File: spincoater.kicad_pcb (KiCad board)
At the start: 2 copper layers, 100 x 60 mm, 1 part, among them U301 TMC4671-ES

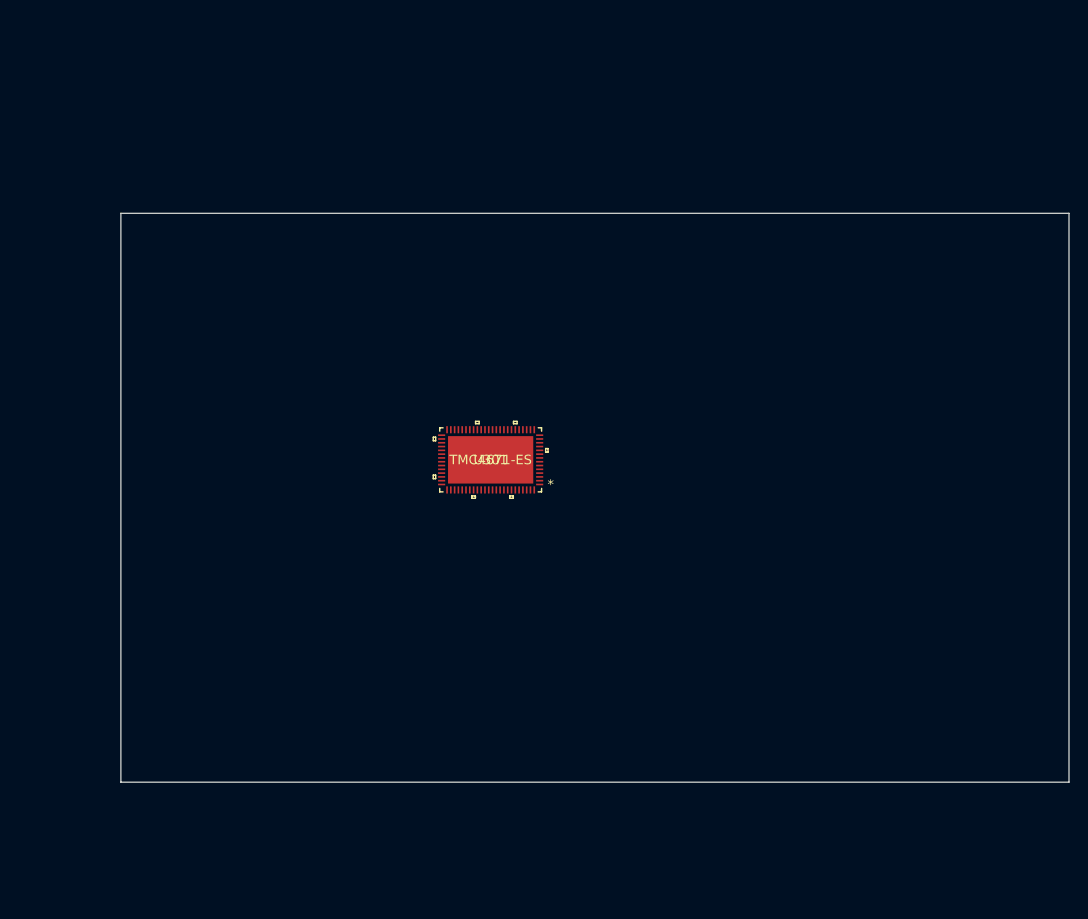
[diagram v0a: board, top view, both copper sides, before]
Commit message: antes de comenzar a rutear
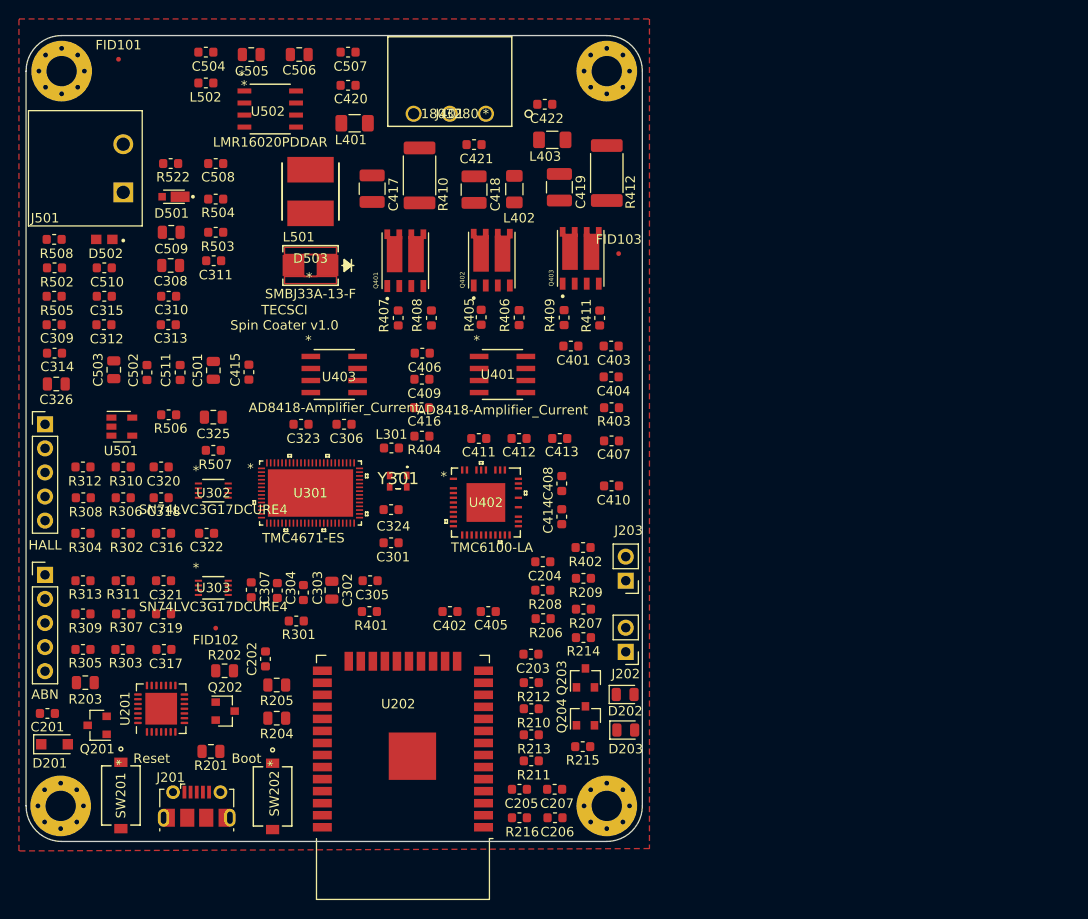
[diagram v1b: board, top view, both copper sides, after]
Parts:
- added C201: 0.1uF/50V/0603, Capacitor_SMD:C_0603_1608Metric, F.Cu at (42.2, 111.8)
- added C202: 0.1uF/50V/0603, Capacitor_SMD:C_0603_1608Metric, F.Cu at (65.2, 106.0)
- added C203: 100nF/50V/0603, Capacitor_SMD:C_0603_1608Metric, F.Cu at (93.2, 105.5)
- added C204: 100nF/50V/0603, Capacitor_SMD:C_0603_1608Metric, F.Cu at (94.5, 95.8)
- added C205: 0.1uF/50V/0603, Capacitor_SMD:C_0603_1608Metric, F.Cu at (92.0, 119.8)
- added C206: 22uF/10V/0603, Capacitor_SMD:C_0603_1608Metric, F.Cu at (95.8, 122.8)
- added C207: 0.1uF/50V/0603, Capacitor_SMD:C_0603_1608Metric, F.Cu at (95.8, 119.8)
- added C301: 100nF/50V/0603, Capacitor_SMD:C_0603_1608Metric, F.Cu at (78.5, 93.8)
- added C302: 4.7uF/16V/0805, Capacitor_SMD:C_0805_2012Metric, F.Cu at (72.2, 98.8)
- added C303: 100nF/50V/0603, Capacitor_SMD:C_0603_1608Metric, F.Cu at (69.2, 99.0)
- added C304: 100nF/50V/0603, Capacitor_SMD:C_0603_1608Metric, F.Cu at (66.5, 98.8)
- added C305: 100nF/50V/0603, Capacitor_SMD:C_0603_1608Metric, F.Cu at (76.3, 97.8)
- added C306: 100nF/50V/0603, Capacitor_SMD:C_0603_1608Metric, F.Cu at (73.5, 81.2)
- added C307: 100nF/50V/0603, Capacitor_SMD:C_0603_1608Metric, F.Cu at (63.8, 98.7)
- added C308: 4.7uF/16V/0805, Capacitor_SMD:C_0805_2012Metric, F.Cu at (55.2, 64.5)
- added C309: 470nF/50V/0603, Capacitor_SMD:C_0603_1608Metric, F.Cu at (43.0, 70.8)
- added C310: 100nF/50V/0603, Capacitor_SMD:C_0603_1608Metric, F.Cu at (55.0, 67.8)
- added C311: 100nF/50V/0603, Capacitor_SMD:C_0603_1608Metric, F.Cu at (59.8, 64.0)
- added C312: 100nF/50V/0603, Capacitor_SMD:C_0603_1608Metric, F.Cu at (48.2, 70.8)
- added C313: 100nF/50V/0603, Capacitor_SMD:C_0603_1608Metric, F.Cu at (55.0, 70.8)
- added C314: 100nF/50V/0603, Capacitor_SMD:C_0603_1608Metric, F.Cu at (43.0, 73.8)
- added C315: 100nF/50V/0603, Capacitor_SMD:C_0603_1608Metric, F.Cu at (48.2, 67.8)
- added C316: 1nF/100V/0603, Capacitor_SMD:C_0603_1608Metric, F.Cu at (54.5, 92.8)
- added C317: 1nF/100V/0603, Capacitor_SMD:C_0603_1608Metric, F.Cu at (54.5, 105.0)
- added C318: 1nF/100V/0603, Capacitor_SMD:C_0603_1608Metric, F.Cu at (54.2, 89.0)
- added C319: 1nF/100V/0603, Capacitor_SMD:C_0603_1608Metric, F.Cu at (54.5, 101.2)
- added C320: 1nF/100V/0603, Capacitor_SMD:C_0603_1608Metric, F.Cu at (54.2, 85.8)
- added C321: 1nF/100V/0603, Capacitor_SMD:C_0603_1608Metric, F.Cu at (54.5, 97.8)
- added C322: 100nF/50V/0603, Capacitor_SMD:C_0603_1608Metric, F.Cu at (59.0, 92.8)
- added C323: 100nF/50V/0603, Capacitor_SMD:C_0603_1608Metric, F.Cu at (69.0, 81.2)
- added C324: 100nF/50V 0603, Capacitor_SMD:C_0603_1608Metric, F.Cu at (78.5, 90.2)
- added C325: 1uF/50V/0805, Capacitor_SMD:C_0805_2012Metric, F.Cu at (59.8, 80.5)
- added C326: 1uF/50V/0805, Capacitor_SMD:C_0805_2012Metric, F.Cu at (43.2, 77.0)
- added C401: 100nF/50v/0603, Capacitor_SMD:C_0603_1608Metric, F.Cu at (97.5, 73.0)
- added C402: 2.2uF/16V/0603, Capacitor_SMD:C_0603_1608Metric, F.Cu at (84.7, 101.0)
- added C403: 2.2uF/16V/0603, Capacitor_SMD:C_0603_1608Metric, F.Cu at (101.7, 73.0)
- added C404: 100nF/50V/0603, Capacitor_SMD:C_0603_1608Metric, F.Cu at (101.7, 76.2)
- added C405: 100nF/50V/0603, Capacitor_SMD:C_0603_1608Metric, F.Cu at (88.8, 101.0)
- added C406: 100nF/50V/0603, Capacitor_SMD:C_0603_1608Metric, F.Cu at (81.8, 73.8)
- added C407: 2.2nF/50V/0603, Capacitor_SMD:C_0603_1608Metric, F.Cu at (101.8, 83.0)
- added C408: 100nF/50V/0603, Capacitor_SMD:C_0603_1608Metric, F.Cu at (96.5, 87.5)
- added C409: 100nF/50V/0603, Capacitor_SMD:C_0603_1608Metric, F.Cu at (81.8, 76.5)
- added C410: 100nF/50V/0603, Capacitor_SMD:C_0603_1608Metric, F.Cu at (101.8, 87.8)
- added C411: 470nF/50V/0603, Capacitor_SMD:C_0603_1608Metric, F.Cu at (87.8, 82.8)
- added C412: 470nF/50V/0603, Capacitor_SMD:C_0603_1608Metric, F.Cu at (92.0, 82.8)
- added C413: 470nF/50V/0603, Capacitor_SMD:C_0603_1608Metric, F.Cu at (96.3, 82.8)
- added C414: 22nF/100V/0603, Capacitor_SMD:C_0603_1608Metric, F.Cu at (96.5, 91.0)
- added C415: 100nF/50V/0603, Capacitor_SMD:C_0603_1608Metric, F.Cu at (63.5, 75.8)
- added C416: 2.2nF/50V/0603, Capacitor_SMD:C_0603_1608Metric, F.Cu at (81.7, 79.5)
- added C417: 10uF/50V/1210, Capacitor_SMD:C_1210_3225Metric, F.Cu at (76.5, 56.4)
- added C418: 10uF/50V/1210, Capacitor_SMD:C_1210_3225Metric, F.Cu at (87.2, 56.5)
- added C419: 10uF/50V/1210, Capacitor_SMD:C_1210_3225Metric, F.Cu at (96.2, 56.2)
- added C420: 1nF/100V/0603, Capacitor_SMD:C_0603_1608Metric, F.Cu at (74.0, 45.5)
- added C421: 1nF/100V/0603, Capacitor_SMD:C_0603_1608Metric, F.Cu at (87.2, 51.8)
- added C422: 1nF/100V/0603, Capacitor_SMD:C_0603_1608Metric, F.Cu at (94.7, 47.5)
- added C501: 10uF/16V/0805, Capacitor_SMD:C_0805_2012Metric, F.Cu at (59.8, 75.6)
- added C502: 10nF/16V/0603, Capacitor_SMD:C_0603_1608Metric, F.Cu at (52.8, 75.8)
- added C503: 10uF/16V/0805, Capacitor_SMD:C_0805_2012Metric, F.Cu at (49.2, 75.5)
- added C504: 100nF/50V/0603, Capacitor_SMD:C_0603_1608Metric, F.Cu at (59.0, 42.0)
- added C505: 2.2uF/50V/0805, Capacitor_SMD:C_0805_2012Metric, F.Cu at (63.8, 42.2)
- added C506: 2.2uF/50V/0805, Capacitor_SMD:C_0805_2012Metric, F.Cu at (68.8, 42.2)
- added C507: 100nF/50V/0603, Capacitor_SMD:C_0603_1608Metric, F.Cu at (74.0, 42.0)
- added C508: 100nF/50V/0603, Capacitor_SMD:C_0603_1608Metric, F.Cu at (60.0, 53.8)
- added C509: 10uF/16V/0805, Capacitor_SMD:C_0805_2012Metric, F.Cu at (55.3, 61.0)
- added C510: 100nF/50V/0603, Capacitor_SMD:C_0603_1608Metric, F.Cu at (48.2, 64.8)
- added C511: 100nF/50V/0603, Capacitor_SMD:C_0603_1608Metric, F.Cu at (56.2, 75.8)
- added D201: PMEG3020EH, Diode_SMD:D_SOD-123F, F.Cu at (43.0, 115.0)
- added D202: LED, LED_SMD:LED_0805_2012Metric, F.Cu at (103.2, 109.8)
- added D203: LED, LED_SMD:LED_0805_2012Metric, F.Cu at (103.2, 113.5)
- added D501: V2PM10HM3, DIODE_MSS1P4-M3:DIODE_MSS1P4-M3, F.Cu at (55.6, 57.2)
- added D502: LTST-C191TBKT-5A, LTST-C191TBKT-5A:LTST-C191TBKT-5A, F.Cu at (48.2, 61.8)
- added D503: SMBJ33A-13-F, SMBJ33A-13-F:SMBJ33A-13-F, F.Cu at (70.0, 64.5)
- added FID101: Fiducial, Fiducial:Fiducial_0.5mm_Mask1mm, F.Cu at (49.8, 42.8)
- added FID102: Fiducial, Fiducial:Fiducial_0.5mm_Mask1mm, F.Cu at (60.0, 102.8)
- added FID103: Fiducial, Fiducial:Fiducial_0.5mm_Mask1mm, F.Cu at (102.5, 63.2)
- added H101: MountingHole_Pad, MountingHole:MountingHole_3.2mm_M3_Pad_Via, F.Cu at (43.8, 44.0)
- added H102: MountingHole_Pad, MountingHole:MountingHole_3.2mm_M3_Pad_Via, F.Cu at (43.6, 121.5)
- added H103: MountingHole_Pad, MountingHole:MountingHole_3.2mm_M3_Pad_Via, F.Cu at (101.2, 121.5)
- added H104: MountingHole_Pad, MountingHole:MountingHole_3.2mm_M3_Pad_Via, F.Cu at (101.2, 44.0)
- added J201: USB_B_Micro, Connector_USB:USB_Micro-B_Molex-105017-0001, F.Cu at (58.0, 121.5)
- added J202: Conn_01x02, Connector_PinHeader_2.54mm:PinHeader_1x02_P2.54mm_Vertical, F.Cu at (103.2, 105.2)
- added J203: Conn_01x02, Connector_PinHeader_2.54mm:PinHeader_1x02_P2.54mm_Vertical, F.Cu at (103.2, 97.8)
- added J301: Conn_01x05, Connector_PinHeader_2.54mm:PinHeader_1x05_P2.54mm_Vertical, F.Cu at (42.0, 81.2)
- added J302: Conn_01x05, Connector_PinHeader_2.54mm:PinHeader_1x05_P2.54mm_Vertical, F.Cu at (42.0, 97.1)
- added J401: 1803280, 1803280:1803280, F.Cu at (88.5, 48.5)
- added J501: 1757242, PHOENIX_1757242:PHOENIX_1757242, F.Cu at (46.2, 54.2)
- added L301: 600R/1A/0603, Inductor_SMD:L_0603_1608Metric, F.Cu at (78.5, 83.8)
- added L401: 50R/12A/1206, Inductor_SMD:L_1206_3216Metric, F.Cu at (74.7, 49.5)
- added L402: 50R/12A/1206, Inductor_SMD:L_1206_3216Metric, F.Cu at (91.5, 56.5)
- added L403: 50R/12A/1206, Inductor_SMD:L_1206_3216Metric, F.Cu at (95.5, 51.2)
- added L501: 15uH/2.5A/VLS6045, INDPM6060X450N:INDPM6060X450N, F.Cu at (70.0, 56.7)
- added L502: 600R/1A/0603, Inductor_SMD:L_0603_1608Metric, F.Cu at (59.0, 45.2)
- added Q201: S8050, Package_TO_SOT_SMD:SOT-23, F.Cu at (47.5, 113.0)
- added Q202: S8050, Package_TO_SOT_SMD:SOT-23, F.Cu at (61.0, 111.5)
- added Q203: 2N7002, Package_TO_SOT_SMD:SOT-23, F.Cu at (99.0, 108.0)
- added Q204: 2N7002, Package_TO_SOT_SMD:SOT-23, F.Cu at (99.0, 112.0)
- added Q401: SI7288DP-T1-GE3, SI7288DP-T1-GE3:TRANS_SI7288DP-T1-GE3, F.Cu at (80.0, 64.0)
- added Q402: SI7288DP-T1-GE3, SI7288DP-T1-GE3:TRANS_SI7288DP-T1-GE3, F.Cu at (89.1, 63.9)
- added Q403: SI7288DP-T1-GE3, SI7288DP-T1-GE3:TRANS_SI7288DP-T1-GE3, F.Cu at (98.5, 63.8)
- added R201: 4.7K/1%/0805, Resistor_SMD:R_0805_2012Metric, F.Cu at (59.5, 115.8)
- added R202: 10K/1%/0805, Resistor_SMD:R_0805_2012Metric, F.Cu at (60.9, 107.2)
- added R203: 10K/1%/0805, Resistor_SMD:R_0805_2012Metric, F.Cu at (46.2, 108.5)
- added R204: 1K/1%/0805, Resistor_SMD:R_0805_2012Metric, F.Cu at (66.4, 112.2)
- added R205: 1K/1%/0805, Resistor_SMD:R_0805_2012Metric, F.Cu at (66.4, 108.8)
- added R206: 1K/1%/0603, Resistor_SMD:R_0603_1608Metric, F.Cu at (94.5, 101.8)
- added R207: 10K/1%/0603, Resistor_SMD:R_0603_1608Metric, F.Cu at (98.8, 100.8)
- added R208: 1K/1%/0603, Resistor_SMD:R_0603_1608Metric, F.Cu at (94.5, 98.8)
- added R209: 10K/1%/0603, Resistor_SMD:R_0603_1608Metric, F.Cu at (98.8, 97.5)
- added R210: 330K/1%/0603, Resistor_SMD:R_0603_1608Metric, F.Cu at (93.3, 111.2)
- added R211: 330K/1%/0603, Resistor_SMD:R_0603_1608Metric, F.Cu at (93.3, 116.8)
- added R212: 10K/1%/0603, Resistor_SMD:R_0603_1608Metric, F.Cu at (93.3, 108.5)
- added R213: 10K/1%/0603, Resistor_SMD:R_0603_1608Metric, F.Cu at (93.3, 114.0)
- added R214: 680/1%/0603, Resistor_SMD:R_0603_1608Metric, F.Cu at (98.8, 103.8)
- added R215: 680/1%/0603, Resistor_SMD:R_0603_1608Metric, F.Cu at (98.7, 115.2)
- added R216: 10K/1%/0603, Resistor_SMD:R_0603_1608Metric, F.Cu at (92.0, 122.8)
- added R301: 10K/1%/0603, Resistor_SMD:R_0603_1608Metric, F.Cu at (68.5, 102.0)
- added R302: 4K7/1%/0603, Resistor_SMD:R_0603_1608Metric, F.Cu at (50.2, 92.8)
- added R303: 4K7/1%/0603, Resistor_SMD:R_0603_1608Metric, F.Cu at (50.2, 105.0)
- added R304: 4K7/1%/0603, Resistor_SMD:R_0603_1608Metric, F.Cu at (46.0, 92.8)
- added R305: 4K7/1%/0603, Resistor_SMD:R_0603_1608Metric, F.Cu at (46.0, 105.0)
- added R306: 4K7/1%/0603, Resistor_SMD:R_0603_1608Metric, F.Cu at (50.2, 89.0)
- added R307: 4K7/1%/0603, Resistor_SMD:R_0603_1608Metric, F.Cu at (50.3, 101.2)
- added R308: 4K7/1%/0603, Resistor_SMD:R_0603_1608Metric, F.Cu at (46.0, 89.0)
- added R309: 4K7/1%/0603, Resistor_SMD:R_0603_1608Metric, F.Cu at (46.0, 101.2)
- added R310: 4K7/1%/0603, Resistor_SMD:R_0603_1608Metric, F.Cu at (50.2, 85.8)
- added R311: 4K7/1%/0603, Resistor_SMD:R_0603_1608Metric, F.Cu at (50.2, 97.8)
- added R312: 4K7/1%/0603, Resistor_SMD:R_0603_1608Metric, F.Cu at (46.0, 85.8)
- added R313: 4K7/1%/0603, Resistor_SMD:R_0603_1608Metric, F.Cu at (46.0, 97.8)
- added R401: 10K/1%/0603, Resistor_SMD:R_0603_1608Metric, F.Cu at (76.2, 101.0)
- added R402: 10K/1%/0603, Resistor_SMD:R_0603_1608Metric, F.Cu at (98.8, 94.2)
- added R403: 1K/1%/0603, Resistor_SMD:R_0603_1608Metric, F.Cu at (101.8, 79.5)
- added R404: 1k/1%/0603, Resistor_SMD:R_0603_1608Metric, F.Cu at (81.8, 82.5)
- added R405: 10R/1%/0603, Resistor_SMD:R_0603_1608Metric, F.Cu at (88.0, 70.0)
- added R406: 10R/1%/0603, Resistor_SMD:R_0603_1608Metric, F.Cu at (92.0, 70.0)
- added R407: 10R/1%/0603, Resistor_SMD:R_0603_1608Metric, F.Cu at (79.2, 70.0)
- added R408: 10R/1%/0603, Resistor_SMD:R_0603_1608Metric, F.Cu at (82.8, 70.0)
- added R409: 10R/1%/0603, Resistor_SMD:R_0603_1608Metric, F.Cu at (96.8, 70.0)
- added R410: 0R005/1%/3W/2512, Resistor_SMD:R_2512_6332Metric, F.Cu at (81.5, 55.0)
- added R411: 10R/1%/0603, Resistor_SMD:R_0603_1608Metric, F.Cu at (100.5, 70.0)
- added R412: 0R005/1%/3W/2512, Resistor_SMD:R_2512_6332Metric, F.Cu at (101.2, 54.8)
- added R502: 220K/1%/0603, Resistor_SMD:R_0603_1608Metric, F.Cu at (43.0, 64.8)
- added R503: 47K/1%/0603, Resistor_SMD:R_0603_1608Metric, F.Cu at (60.0, 61.0)
- added R504: 270K/1%/0603, Resistor_SMD:R_0603_1608Metric, F.Cu at (60.0, 57.5)
- added R505: 10K/1%/0603, Resistor_SMD:R_0603_1608Metric, F.Cu at (43.0, 67.8)
- added R506: 1K/1%/0603, Resistor_SMD:R_0603_1608Metric, F.Cu at (55.0, 80.2)
- added R507: 1K/1%/0603, Resistor_SMD:R_0603_1608Metric, F.Cu at (59.8, 84.0)
- added R508: 10K/1%/0603, Resistor_SMD:R_0603_1608Metric, F.Cu at (43.0, 61.8)
- added R522: 33K/1%/0603, Resistor_SMD:R_0603_1608Metric, F.Cu at (55.2, 53.8)
- added SW201: Reset, KSR223GLFG:KSR223GLFG, F.Cu at (50.0, 116.9)
- added SW202: Boot, KSR223GLFG:KSR223GLFG, F.Cu at (66.0, 117.0)
- added U201: CP2102N-A01-GQFN28, Package_DFN_QFN:QFN-28-1EP_5x5mm_P0.5mm_EP3.35x3.35mm, F.Cu at (54.2, 111.2)
- added U202: ESP32-WROOM-32D, RF_Module:ESP32-WROOM-32, F.Cu at (79.8, 115.5)
- added U302: SN74LVC3G17DCURE4, SN74LVC3G17DCURE4:SN74LVC3G17DCURE4, F.Cu at (59.8, 88.2)
- added U303: SN74LVC3G17DCURE4, SN74LVC3G17DCURE4:SN74LVC3G17DCURE4, F.Cu at (59.8, 98.5)
- added U401: AD8418-Amplifier_Current, AD8418WBRZ-RL:AD8418WBRZ-RL, F.Cu at (90.2, 76.0)
- added U402: TMC6100-LA, TMC6100-LA:TMC6100-LA, F.Cu at (88.5, 89.5)
- added U403: AD8418-Amplifier_Current, AD8418WBRZ-RL:AD8418WBRZ-RL, F.Cu at (72.5, 76.0)
- added U501: LP2985-3.3, Package_TO_SOT_SMD:SOT-23-5, F.Cu at (50.1, 81.5)
- added U502: LMR16020PDDAR, LMR16020PDDAR:LMR16020PDDAR, F.Cu at (65.8, 48.0)
- added Y301: MC2016K25.0000C16ESH, MC2016K250000C16ESH:MC2016K250000C16ESH, F.Cu at (79.2, 87.2)
- U301: footprint footprints:TMC4671-ES -> TMC4671-LA:TMC4671-LA
- moved U301 19.3 mm to (70.0, 88.5), turned to 0 degrees
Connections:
- U301 pad 1: (no net) -> Net-(U301-Pad1)
- U301 pad 11: (no net) -> Net-(U301-Pad11)
- U301 pad 12: (no net) -> Net-(U301-Pad12)
- U301 pad 13: (no net) -> +3V3
- U301 pad 14: (no net) -> GND
- U301 pad 15: (no net) -> Net-(C304-Pad1)
- U301 pad 16: Net-(U301-Pad16) -> CUR_U
- U301 pad 17: Net-(U301-Pad17) -> +2.5V_REF
- U301 pad 18: Net-(U301-Pad18) -> CUR_W
- U301 pad 19: Net-(U301-Pad19) -> +2.5V_REF
- U301 pad 2: (no net) -> +3V3
- U301 pad 20: Net-(U301-Pad20) -> ADC_+24
- U301 pad 23: (no net) -> +5V
- U301 pad 24: (no net) -> GND
- U301 pad 3: (no net) -> GND
- U301 pad 32: Net-(U301-Pad32) -> EN_6100
- U301 pad 39: Net-(U301-Pad39) -> UH
- U301 pad 4: (no net) -> Net-(U301-Pad4)
- U301 pad 40: Net-(U301-Pad40) -> UL
- U301 pad 41: Net-(U301-Pad41) -> VH
- U301 pad 42: Net-(U301-Pad42) -> VL
- U301 pad 43: (no net) -> +3V3
- U301 pad 44: (no net) -> GND
- U301 pad 45: (no net) -> Net-(C305-Pad1)
- U301 pad 46: Net-(U301-Pad46) -> WH
- U301 pad 47: Net-(U301-Pad47) -> WL
- U301 pad 5: (no net) -> Net-(U301-Pad5)
- U301 pad 52: (no net) -> +3V3
- U301 pad 53: (no net) -> GND
- U301 pad 54: Net-(U301-Pad54) -> GND
- U301 pad 55: Net-(U301-Pad55) -> EN_4671
- U301 pad 59: Net-(U301-Pad59) -> GND
- U301 pad 6: Net-(U301-Pad6) -> CS_4671
- U301 pad 60: Net-(U301-Pad60) -> GND
- U301 pad 61: (no net) -> +3V3
- U301 pad 62: (no net) -> GND
- U301 pad 63: (no net) -> Net-(C306-Pad1)
- U301 pad 7: Net-(U301-Pad7) -> SPI_SCK
- U301 pad 70: (no net) -> Net-(U301-Pad70)
- U301 pad 71: (no net) -> Net-(U301-Pad71)
- U301 pad 72: (no net) -> +3V3
- U301 pad 73: (no net) -> GND
- U301 pad 74: (no net) -> Net-(U301-Pad74)
- U301 pad 75: (no net) -> Net-(U301-Pad75)
- U301 pad 76: (no net) -> Net-(U301-Pad76)
- U301 pad 8: Net-(U301-Pad8) -> SPI_MOSI
- U301 pad 9: (no net) -> SPI_MISO
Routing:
- added copper zone on F.Cu, net GND
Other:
- board size 100 x 60 mm -> 65 x 85 mm
- copper layers 2 -> 4
- board text added: "ABN"
- board text added: "HALL"
- board text added: "TECSCI Spin Coater v1.0"
